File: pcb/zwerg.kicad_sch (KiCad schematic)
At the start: 57 parts, among them J1 AudioJack4, U1 RP2040-Matrix

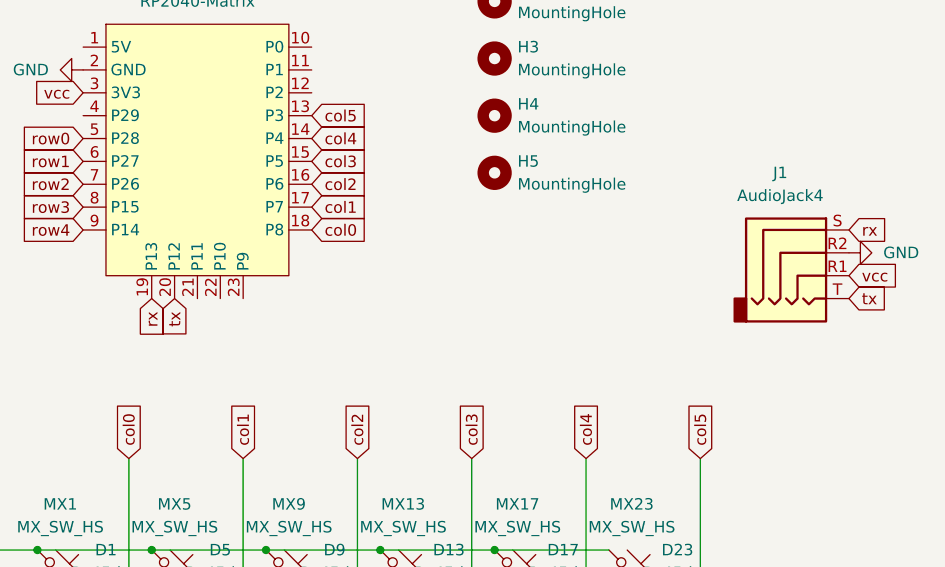
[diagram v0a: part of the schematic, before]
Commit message: updated pcb and case v1.0
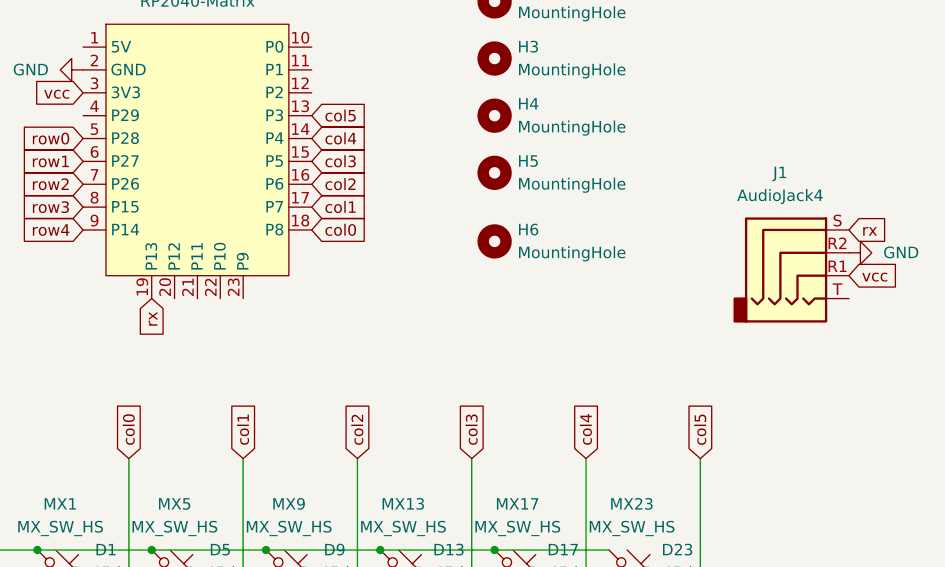
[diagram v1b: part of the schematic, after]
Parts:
- added H6: MountingHole, MountingHole:MountingHole_2.2mm_M2_DIN965_Pad_TopBottom, symbol Mechanical:MountingHole
- D1, D10, D11, D12, D13, D14, D15, D16, D17, D18, D19, D2, D20, D21, D22, D23, D24, D25, D3, D4, D5, D6, D7, D8, D9: footprint kbd:D3_TH_SMD -> zwerg:D3_TH_SMD
- H1, H2, H3, H4, H5: footprint MountingHole:MountingHole_2.2mm_M2_DIN965_Pad_TopBottom -> MountingHole:MountingHole_4.3mm_M4
- U1: footprint PCM_marbastlib-xp-promicroish:RP2040-Matrix_AC -> zwerg:RP2040-Matrix_fb
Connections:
- net tx: no longer names the net of U1.20 (P12)
- net tx: no longer J1.T
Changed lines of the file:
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@@
 		)
 	)
-	(global_label "tx"
-		(shape input)
-		(at 78.74 73.66 270)
-		(fields_autoplaced yes)
-		(effects
-			(font
-				(size 1.27 1.27)
-			)
-			(justify right)
-		)
-		(property "Intersheetrefs" "${INTERSHEET_REFS}"
-			(at 78.74 78.399 90)
-			(effects
-				(font
-					(size 1.27 1.27)
-				)
-				(justify right)
-				(hide yes)
-			)
-		)
-	)
 	(global_label "col5"
 		(shape input)
@@
 		)
 	)
-	(global_label "tx"
-		(shape input)
-		(at 153.67 73.66 0)
-		(fields_autoplaced yes)
-		(effects
-			(font
-				(size 1.27 1.27)
-			)
-			(justify left)
-		)
-		(property "Intersheetrefs" "${INTERSHEET_REFS}"
-			(at 158.409 73.66 0)
-			(effects
-				(font
-					(size 1.27 1.27)
-				)
-				(justify left)
-				(hide yes)
-			)
-		)
-	)
 	(global_label "col2"
 		(shape input)
@@
 			)
 		)
-		(property "Footprint" "kbd:D3_TH_SMD"
+		(property "Footprint" "zwerg:D3_TH_SMD"
 			(at 109.22 147.32 0)
 			(effects
@@
 			)
 		)
-		(property "Footprint" "kbd:D3_TH_SMD"
+		(property "Footprint" "zwerg:D3_TH_SMD"
 			(at 71.12 134.62 0)
 			(effects
@@
 			)
 		)
-		(property "Footprint" "kbd:D3_TH_SMD"
+		(property "Footprint" "zwerg:D3_TH_SMD"
 			(at 96.52 121.92 0)
 			(effects
@@
 			)
 		)
-		(property "Footprint" "kbd:D3_TH_SMD"
+		(property "Footprint" "zwerg:D3_TH_SMD"
 			(at 121.92 147.32 0)
 			(effects
@@
 			)
 		)
-		(property "Footprint" "kbd:D3_TH_SMD"
+		(property "Footprint" "zwerg:D3_TH_SMD"
 			(at 134.62 160.02 0)
 			(effects
@@
 			)
 		)
-		(property "Footprint" "PCM_marbastlib-xp-promicroish:RP2040-Matrix_AC"
+		(property "Footprint" "zwerg:RP2040-Matrix_fb"
 			(at 81.28 90.17 0)
 			(effects
@@
 			)
 		)
-		(property "Footprint" "kbd:D3_TH_SMD"
+		(property "Footprint" "zwerg:D3_TH_SMD"
 			(at 121.92 160.02 0)
 			(effects
@@
 			)
 		)
-		(property "Footprint" "kbd:D3_TH_SMD"
+		(property "Footprint" "zwerg:D3_TH_SMD"
 			(at 71.12 147.32 0)
 			(effects
@@
 			)
 		)
-		(property "Footprint" "kbd:D3_TH_SMD"
+		(property "Footprint" "zwerg:D3_TH_SMD"
 			(at 83.82 121.92 0)
 			(effects
@@
 			)
 		)
-		(property "Footprint" "kbd:D3_TH_SMD"
+		(property "Footprint" "zwerg:D3_TH_SMD"
 			(at 83.82 134.62 0)
 			(effects
@@
 	)
 	(symbol
+		(lib_id "Mechanical:MountingHole")
+		(at 114.3 67.31 0)
+		(unit 1)
+		(exclude_from_sim yes)
+		(in_bom no)
+		(on_board yes)
+		(dnp no)
+		(fields_autoplaced yes)
+		(property "Reference" "H6"
+			(at 116.84 66.0399 0)
+			(effects
+				(font
+					(size 1.27 1.27)
+				)
+				(justify left)
+			)
+		)
+		(property "Value" "MountingHole"
+			(at 116.84 68.5799 0)
+			(effects
+				(font
+					(size 1.27 1.27)
+				)
+				(justify left)
+			)
+		)
+		(property "Footprint" "MountingHole:MountingHole_2.2mm_M2_DIN965_Pad_TopBottom"
+			(at 114.3 67.31 0)
+			(effects
+				(font
+					(size 1.27 1.27)
+				)
+				(hide yes)
+			)
+		)
+		(property "Datasheet" "~"
+			(at 114.3 67.31 0)
+			(effects
+				(font
+					(size 1.27 1.27)
+				)
+				(hide yes)
+			)
+		)
+		(property "Description" "Mounting Hole without connection"
+			(at 114.3 67.31 0)
+			(effects
+				(font
+					(size 1.27 1.27)
+				)
+				(hide yes)
+			)
+		)
+		(instances
+			(project "zwerg"
+				(path "/fe8df7b9-368d-4c77-a717-5363f47564e5"
+					(reference "H6")
+					(unit 1)
+				)
+			)
+		)
+	)
+	(symbol
 		(lib_id "PCM_marbastlib-mx:MX_SW_HS_CPG151101S11")
 		(at 116.84 142.24 0)
@@
 			)
 		)
-		(property "Footprint" "kbd:D3_TH_SMD"
+		(property "Footprint" "zwerg:D3_TH_SMD"
 			(at 96.52 109.22 0)
 			(effects
@@
 			)
 		)
-		(property "Footprint" "MountingHole:MountingHole_2.2mm_M2_DIN965_Pad_TopBottom"
+		(property "Footprint" "MountingHole:MountingHole_4.3mm_M4"
 			(at 114.3 59.69 0)
 			(effects
@@
 			)
 		)
-		(property "Footprint" "kbd:D3_TH_SMD"
+		(property "Footprint" "zwerg:D3_TH_SMD"
 			(at 134.62 134.62 0)
 			(effects
@@
 			)
 		)
-		(property "Footprint" "MountingHole:MountingHole_2.2mm_M2_DIN965_Pad_TopBottom"
+		(property "Footprint" "MountingHole:MountingHole_4.3mm_M4"
 			(at 114.3 46.99 0)
 			(effects
@@
 			)
 		)
-		(property "Footprint" "kbd:D3_TH_SMD"
+		(property "Footprint" "zwerg:D3_TH_SMD"
 			(at 109.22 134.62 0)
 			(effects
@@
 			)
 		)
-		(property "Footprint" "kbd:D3_TH_SMD"
+		(property "Footprint" "zwerg:D3_TH_SMD"
 			(at 96.52 134.62 0)
 			(effects
@@
 			)
 		)
-		(property "Footprint" "MountingHole:MountingHole_2.2mm_M2_DIN965_Pad_TopBottom"
+		(property "Footprint" "MountingHole:MountingHole_4.3mm_M4"
 			(at 114.3 53.34 0)
 			(effects
@@
 			)
 		)
-		(property "Footprint" "kbd:D3_TH_SMD"
+		(property "Footprint" "zwerg:D3_TH_SMD"
 			(at 121.92 121.92 0)
 			(effects
@@
 			)
 		)
-		(property "Footprint" "kbd:D3_TH_SMD"
+		(property "Footprint" "zwerg:D3_TH_SMD"
 			(at 71.12 109.22 0)
 			(effects
@@
 			)
 		)
-		(property "Footprint" "kbd:D3_TH_SMD"
+		(property "Footprint" "zwerg:D3_TH_SMD"
 			(at 121.92 109.22 0)
 			(effects
@@
 			)
 		)
-		(property "Footprint" "kbd:D3_TH_SMD"
+		(property "Footprint" "zwerg:D3_TH_SMD"
 			(at 83.82 109.22 0)
 			(effects
@@
 			)
 		)
-		(property "Footprint" "kbd:D3_TH_SMD"
+		(property "Footprint" "zwerg:D3_TH_SMD"
 			(at 96.52 147.32 0)
 			(effects
@@
 			)
 		)
-		(property "Footprint" "MountingHole:MountingHole_2.2mm_M2_DIN965_Pad_TopBottom"
+		(property "Footprint" "MountingHole:MountingHole_4.3mm_M4"
 			(at 114.3 40.64 0)
 			(effects
@@
 			)
 		)
-		(property "Footprint" "kbd:D3_TH_SMD"
+		(property "Footprint" "zwerg:D3_TH_SMD"
 			(at 71.12 121.92 0)
 			(effects
@@
 			)
 		)
-		(property "Footprint" "MountingHole:MountingHole_2.2mm_M2_DIN965_Pad_TopBottom"
+		(property "Footprint" "MountingHole:MountingHole_4.3mm_M4"
 			(at 114.3 34.29 0)
 			(effects
@@
 			)
 		)
-		(property "Footprint" "kbd:D3_TH_SMD"
+		(property "Footprint" "zwerg:D3_TH_SMD"
 			(at 121.92 134.62 0)
 			(effects
@@
 			)
 		)
-		(property "Footprint" "kbd:D3_TH_SMD"
+		(property "Footprint" "zwerg:D3_TH_SMD"
 			(at 83.82 147.32 0)
 			(effects
@@
 			)
 		)
-		(property "Footprint" "kbd:D3_TH_SMD"
+		(property "Footprint" "zwerg:D3_TH_SMD"
 			(at 109.22 121.92 0)
 			(effects
@@
 			)
 		)
-		(property "Footprint" "kbd:D3_TH_SMD"
+		(property "Footprint" "zwerg:D3_TH_SMD"
 			(at 134.62 109.22 0)
 			(effects
@@
 			)
 		)
-		(property "Footprint" "kbd:D3_TH_SMD"
+		(property "Footprint" "zwerg:D3_TH_SMD"
 			(at 134.62 121.92 0)
 			(effects
@@
 			)
 		)
-		(property "Footprint" "kbd:D3_TH_SMD"
+		(property "Footprint" "zwerg:D3_TH_SMD"
 			(at 109.22 109.22 0)
 			(effects
